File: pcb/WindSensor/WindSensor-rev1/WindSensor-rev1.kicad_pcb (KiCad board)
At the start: 2 copper layers, 20 x 20 mm, 17 parts, among them J1 Conn_I2C_Molex_705450003, U1 SDP320x21, U2 SDP320x22, U3 SDP320x23, U4 LP5814DRLR

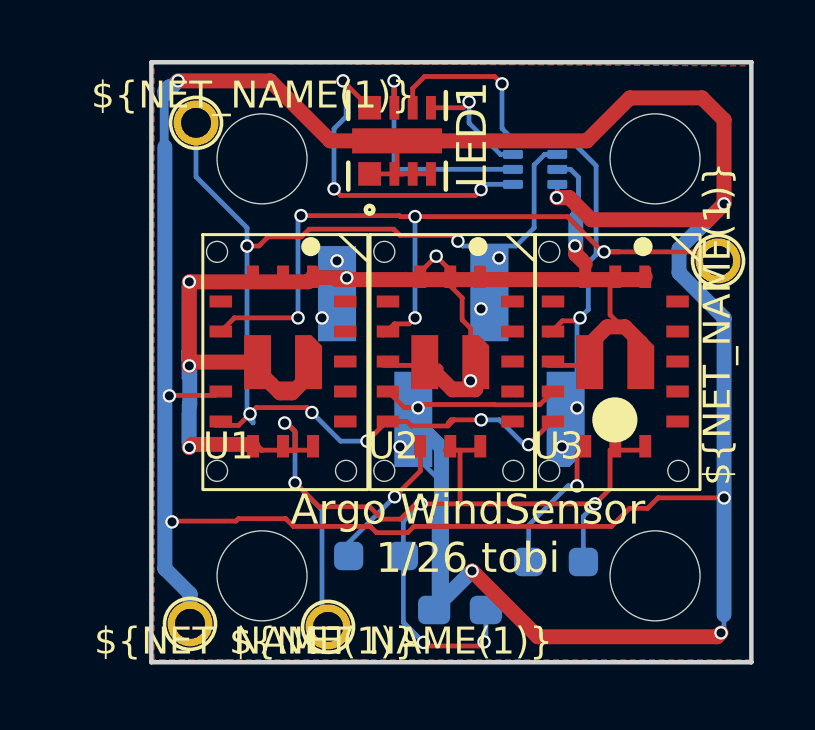
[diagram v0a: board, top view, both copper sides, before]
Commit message: first steps to housing model. adjusted PCB layout slightly. fixed rules
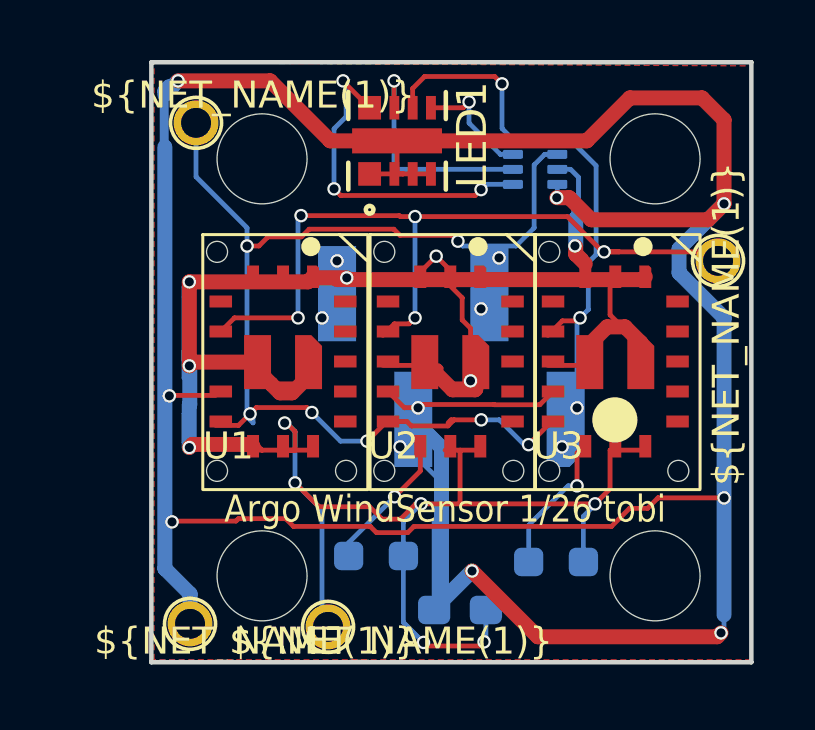
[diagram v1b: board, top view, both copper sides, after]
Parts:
- gave numbers to parts that had none: 4
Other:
- rule pad_to_mask_clearance: 0 -> 0.01
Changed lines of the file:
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@@
 			(dielectric_constraints no)
 		)
-		(pad_to_mask_clearance 0)
+		(pad_to_mask_clearance 0.01)
 		(solder_mask_min_width 0.25)
 		(allow_soldermask_bridges_in_footprints no)
@@
 		)
 		(embedded_fonts no)
-		(model "$(WINDSENSOR_3D)/Sensirion_Differential_Pressure_Sensors_SDP3x_STEP_file.step"
+		(model "3d_models/Sensirion_Differential_Pressure_Sensors_SDP3x_STEP_file.step"
 			(opacity 0.7800)
 			(offset
@@
 		(sheetname "/")
 		(sheetfile "WindSensor-rev1.kicad_sch")
-		(attr exclude_from_pos_files)
+		(attr exclude_from_pos_files exclude_from_bom)
 		(fp_circle
 			(center 0 0)
@@
 		(sheetname "/")
 		(sheetfile "WindSensor-rev1.kicad_sch")
-		(attr exclude_from_pos_files)
+		(attr exclude_from_pos_files exclude_from_bom)
 		(fp_circle
 			(center 0 0)
@@
 		)
 		(fp_text user "${NET_NAME(1)}"
-			(at 0.5 2.1 90)
+			(at 0.8 2.1 90)
 			(unlocked yes)
 			(layer "F.SilkS")
@@
 		)
 		(embedded_fonts no)
-		(model "$(WINDSENSOR_3D)/Sensirion_Differential_Pressure_Sensors_SDP3x_STEP_file.step"
+		(model "3d_models/Sensirion_Differential_Pressure_Sensors_SDP3x_STEP_file.step"
 			(opacity 0.7800)
 			(offset
@@
 		)
 		(embedded_fonts no)
-		(model "$(WINDSENSOR_3D)/Sensirion_Differential_Pressure_Sensors_SDP3x_STEP_file.step"
+		(model "3d_models/Sensirion_Differential_Pressure_Sensors_SDP3x_STEP_file.step"
 			(opacity 0.7800)
 			(offset
@@
 		(layer "F.Cu")
 		(at 88.5 79.4)
-		(property "Reference" ""
+		(property "Reference" "H1"
 			(at 0 0 0)
 			(layer "F.SilkS")
+			(hide yes)
 			(effects
 				(font
@@
 			(at 0 0 0)
 			(layer "F.Fab")
+			(hide yes)
 			(effects
 				(font
@@
 			)
 		)
+		(attr through_hole board_only exclude_from_bom)
 		(pad "" np_thru_hole circle
 			(at 0 0)
@@
 		(layer "F.Cu")
 		(at 101.6 93.3)
-		(property "Reference" ""
+		(property "Reference" "H4"
 			(at 0 0 0)
 			(layer "F.SilkS")
+			(hide yes)
 			(effects
 				(font
@@
 			(at 0 0 0)
 			(layer "F.Fab")
+			(hide yes)
 			(effects
 				(font
@@
 			)
 		)
+		(attr through_hole board_only exclude_from_bom)
 		(pad "" np_thru_hole circle
 			(at 0 0)
@@
 		(sheetname "/")
 		(sheetfile "WindSensor-rev1.kicad_sch")
-		(attr exclude_from_pos_files)
+		(attr exclude_from_pos_files exclude_from_bom)
 		(fp_circle
 			(center 0 0)
@@
 		(layer "F.Cu")
 		(at 101.6 79.4)
-		(property "Reference" ""
+		(property "Reference" "H2"
 			(at 0 0 0)
 			(layer "F.SilkS")
+			(hide yes)
 			(effects
 				(font
@@
 			(at 0 0 0)
 			(layer "F.Fab")
+			(hide yes)
 			(effects
 				(font
@@
 			)
 		)
+		(attr through_hole board_only exclude_from_bom)
 		(pad "" np_thru_hole circle
 			(at 0 0)
@@
 		(sheetname "/")
 		(sheetfile "WindSensor-rev1.kicad_sch")
-		(attr exclude_from_pos_files)
+		(attr exclude_from_pos_files exclude_from_bom)
 		(fp_circle
 			(center 0 0)
@@
 		)
 		(embedded_fonts no)
-		(model "$(WINDSENSOR_3D)/599-2310_DIA.step"
+		(model "./3d_models/599-2310_DIA.step"
 			(offset
 				(xyz 0 0 0)
@@
 		(layer "F.Cu")
 		(at 88.5 93.3)
-		(property "Reference" ""
+		(property "Reference" "H3"
 			(at 0 0 0)
 			(layer "F.SilkS")
+			(hide yes)
 			(effects
 				(font
@@
 			(at 0 0 0)
 			(layer "F.Fab")
+			(hide yes)
 			(effects
 				(font
@@
 			)
 		)
+		(attr through_hole board_only exclude_from_bom)
 		(pad "" np_thru_hole circle
 			(at 0 0)
@@
 		(tags "resistor handsolder")
 		(property "Reference" "R1"
-			(at -0.8 1.2 180)
+			(at 0 1.3625 180)
 			(layer "B.SilkS")
 			(effects
@@
 		(tags "capacitor handsolder")
 		(property "Reference" "C1"
-			(at -2.3 0.7625 180)
+			(at -2.6 0.9625 180)
 			(layer "B.SilkS")
 			(effects
@@
 		(tags "resistor handsolder")
 		(property "Reference" "R2"
-			(at -0.1 1.3 180)
+			(at 0.1 1.4625 180)
 			(layer "B.SilkS")
 			(effects
@@
 		)
 		(embedded_fonts no)
-		(model "$(WINDSENSOR_3D)/LP5814DRLR--3DModel-STEP-269445.STEP"
+		(model "3d_models/LP5814DRLR--3DModel-STEP-269445.STEP"
 			(offset
 				(xyz 0 0 0)
@@
 		)
 		(embedded_fonts no)
-		(model "$(WINDSENSOR_3D)/0740990604.stp"
+		(model "3d_models/0740990604.stp"
 			(offset
 				(xyz 0 -0.5 7)
@@
 		(layer "Edge.Cuts")
 	)
-	(gr_text "Argo WindSensor\n1/26 tobi"
-		(at 95.36 93.29 0)
+	(gr_text "Argo WindSensor 1/26 tobi"
+		(at 94.6 91.6 0)
 		(layer "F.SilkS")
 		(effects
 			(font
-				(size 1 1)
+				(size 0.9 0.8)
 				(thickness 0.15)
 			)
@@
 	)
 	(gr_text "Argo WindSensor\n1/26 tobi"
-		(at 88.333 86.7515 90)
+		(at 87.9 86.7515 90)
 		(layer "B.SilkS")
 		(effects
@@
 					(thickness 0.15)
 				)
-				(justify mirror)
 			)
 		)
@@
 					(thickness 0.15)
 				)
-				(justify mirror)
 			)
 		)
@@
 					(thickness 0.15)
 				)
-				(justify mirror)
 			)
 		)
@@
 					(thickness 0.15)
 				)
-				(justify mirror)
 			)
 		)
